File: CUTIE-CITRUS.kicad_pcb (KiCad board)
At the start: 2 copper layers, 78.5 x 78.5 mm, 72 parts, among them J1 F32Q-1A7H1-11022, J2 F32Q-1A7H1-11022, J3 Bus_M.2_Socket_M, P1 ERM8-025-01-L-D-RA-K-TR, U1 AP3441SHE-7B, U2 ASEK-32.768KHZ-L-R-T, U3 ICM-42688-P, U5 MCP98243, U6 MCP98243, U7 MCP2518FD-xQBB, U8 TCAN334

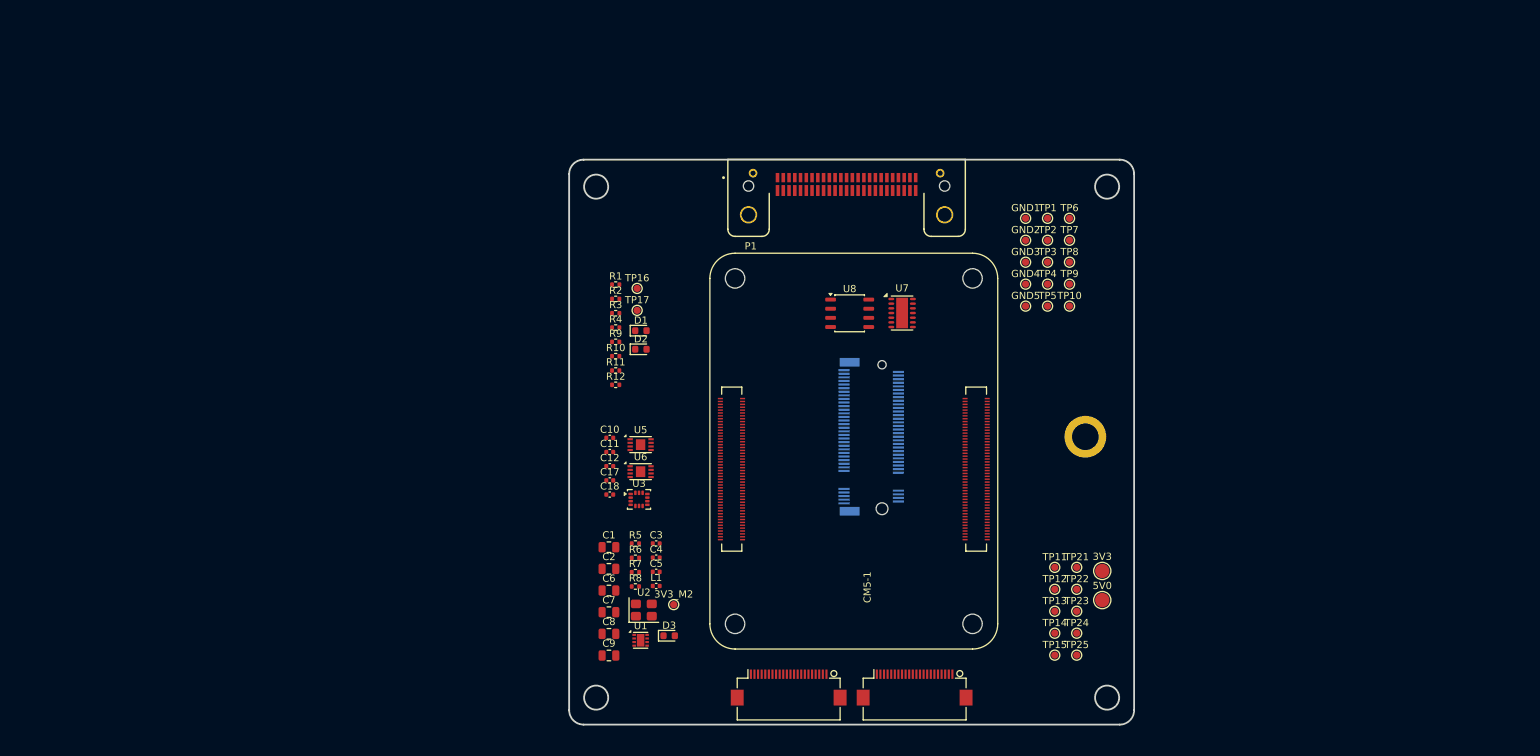
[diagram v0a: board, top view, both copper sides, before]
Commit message: starting layout
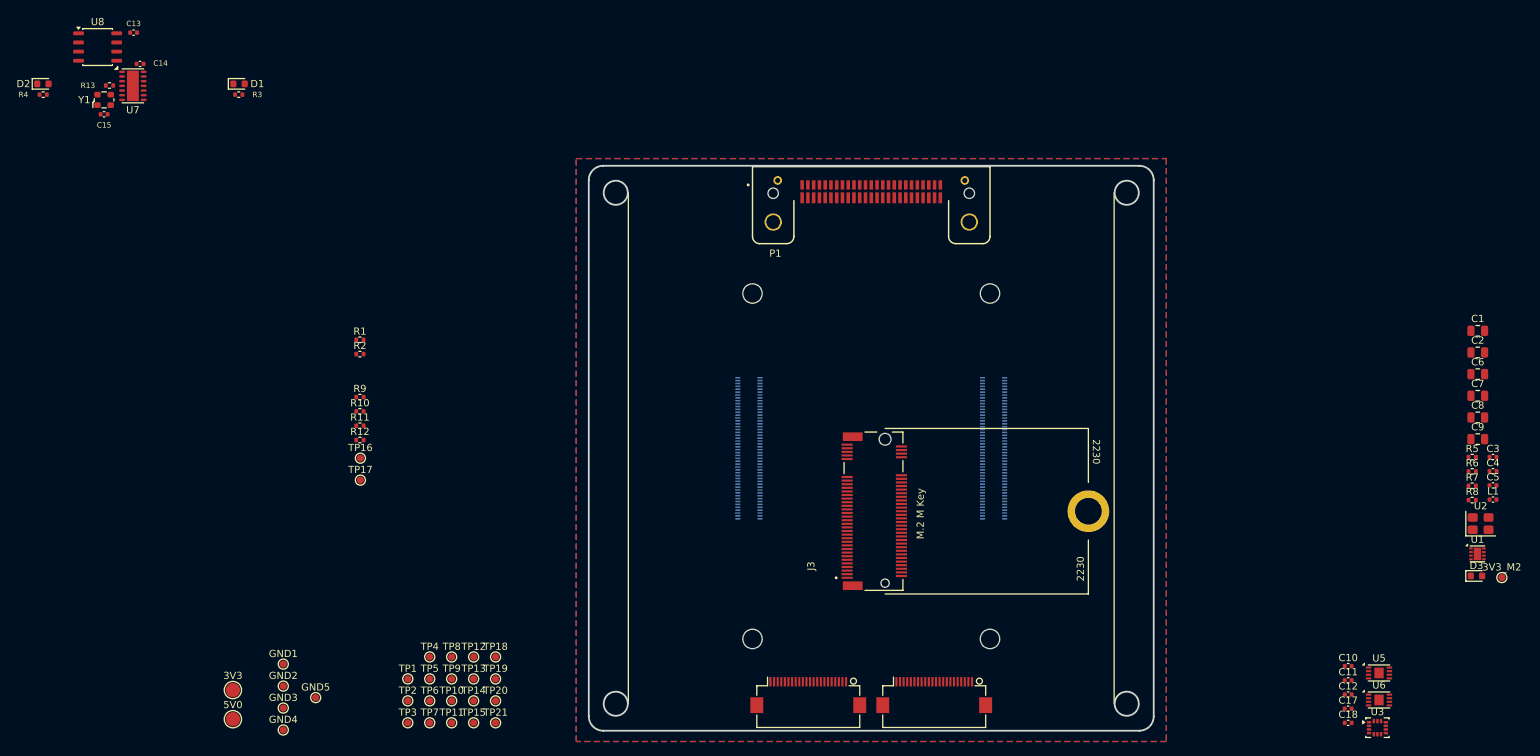
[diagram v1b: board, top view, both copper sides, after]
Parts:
- removed TP22, TP23, TP24, TP25: TestPoint, TestPoint:TestPoint_Pad_D1.0mm
- added C13: 0.1uF, Capacitor_SMD:C_0402_1005Metric, F.Cu at (47.5, 38.5)
- added C14: 0.1uF, Capacitor_SMD:C_0402_1005Metric, F.Cu at (48.4, 42.8)
- added C15: 0.1uF, Capacitor_SMD:C_0402_1005Metric, F.Cu at (43.4, 49.8)
- added R13: 2.2K 1%, Resistor_SMD:R_0402_1005Metric, F.Cu at (44.1, 45.8)
- added TP18: TestPoint, TestPoint:TestPoint_Pad_D1.0mm, F.Cu at (97.8, 125.2)
- added TP19: TestPoint, TestPoint:TestPoint_Pad_D1.0mm, F.Cu at (97.8, 128.3)
- added TP20: TestPoint, TestPoint:TestPoint_Pad_D1.0mm, F.Cu at (97.8, 131.3)
- added Y1: ECS-2520MV-200-BN-TR, Oscillator:Oscillator_SMD_ECS_2520MV-xxx-xx-4Pin_2.5x2.0mm, F.Cu at (43.4, 47.8)
- CM5-1: moved to B.Cu
- J3: moved to F.Cu
- moved C1 124.4 mm to (234.3, 79.9)
- moved C2 124.4 mm to (234.3, 82.9)
- moved C6 124.4 mm to (234.3, 86.0)
- moved C7 124.4 mm to (234.3, 89.0)
- moved C8 124.4 mm to (234.3, 92.0)
- moved C9 124.4 mm to (234.3, 95.0)
- moved 3V3 121.9 mm to (61.3, 129.8)
- moved 5V0 121.9 mm to (61.3, 133.9)
- moved GND2 120.3 mm to (68.3, 129.3)
- moved GND1 120.3 mm to (68.3, 126.2)
- moved GND3 120.3 mm to (68.3, 132.3)
- moved GND4 120.3 mm to (68.3, 135.4)
- moved C3 116.9 mm to (236.4, 97.5)
- moved C4 116.9 mm to (236.4, 99.4)
- moved C5 116.9 mm to (236.4, 101.4)
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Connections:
- net Net-(U7-RXCAN) renamed /CM5/RXCAN
- net Net-(U7-TXCAN) renamed /CM5/TXCAN
- 3V3 pad 1: /Cameras/3V3 -> /CM5/3V3
- C10 pad 1: /Cameras/3V3 -> /CM5/3V3
- C11 pad 1: /Cameras/3V3 -> /CM5/3V3
- C12 pad 1: /Cameras/3V3 -> /CM5/3V3
- C17 pad 1: /Cameras/3V3 -> /CM5/3V3
- C18 pad 1: /Cameras/3V3 -> /CM5/3V3
- CM5-1 pad 128: unconnected-(CM5-1B-USB3-0-RX_N-Pad128) -> /Backplane Connector/USB3.RX_N
- CM5-1 pad 130: unconnected-(CM5-1B-USB3-0-RX_P-Pad130) -> /Backplane Connector/USB3.RX_P
- CM5-1 pad 134: unconnected-(CM5-1B-USB3-0-D_P-Pad134) -> /Backplane Connector/USB3.D_P
- CM5-1 pad 136: unconnected-(CM5-1B-USB3-0-D_N-Pad136) -> /Backplane Connector/USB3.D_N
- CM5-1 pad 140: unconnected-(CM5-1B-USB3-0-TX_N-Pad140) -> /Backplane Connector/USB3.TX_N
- CM5-1 pad 142: unconnected-(CM5-1B-USB3-0-TX_P-Pad142) -> /Backplane Connector/USB3.TX_P
- CM5-1 pad 157: /Backplane Connector/USB3.RX_N -> unconnected-(CM5-1B-USB3-1-RX_N-Pad157)
- CM5-1 pad 159: /Backplane Connector/USB3.RX_P -> unconnected-(CM5-1B-USB3-1-RX_P-Pad159)
- CM5-1 pad 163: /Backplane Connector/USB3.D_P -> unconnected-(CM5-1B-USB3-1-D_P-Pad163)
- CM5-1 pad 165: /Backplane Connector/USB3.D_N -> unconnected-(CM5-1B-USB3-1-D_N-Pad165)
- CM5-1 pad 169: /Backplane Connector/USB3.TX_N -> unconnected-(CM5-1B-USB3-1-TX_N-Pad169)
- CM5-1 pad 171: /Backplane Connector/USB3.TX_P -> unconnected-(CM5-1B-USB3-1-TX_P-Pad171)
- CM5-1 pad 194: GND -> /CM5/DPHY1.D3_N
- CM5-1 pad 196: GND -> /CM5/DPHY1.D3_P
- CM5-1 pad 25: unconnected-(CM5-1A-GPIO21-Pad25) -> /CM5/SPI1.SCLK
- CM5-1 pad 26: unconnected-(CM5-1A-GPIO19-Pad26) -> /CM5/SPI1.MISO
- CM5-1 pad 27: unconnected-(CM5-1A-GPIO20-Pad27) -> /CM5/SPI1.MOSI
- CM5-1 pad 28: unconnected-(CM5-1A-GPIO13-Pad28) -> /CM5/I2C2.SDA
- CM5-1 pad 30: unconnected-(CM5-1A-GPIO6-Pad30) -> /CM5/GPIO/SPI3.MOSI
- CM5-1 pad 31: unconnected-(CM5-1A-GPIO12-Pad31) -> /CM5/I2C2.SDA
- CM5-1 pad 34: /CM5/I2C2.SCL -> /CM5/GPIO/SPI3.MISO
- CM5-1 pad 35: /CM5/I2C1.SCL -> /Backplane Connector/SPI2.MISO
- CM5-1 pad 36: /CM5/I2C1.SDA -> /Backplane Connector/SPI2.CS0n
- CM5-1 pad 37: /CM5/SPI0.CS1n -> /CM5/GPIO/SPI3.SCLK
- CM5-1 pad 38: /CM5/SPI0.SCLK -> /CM5/I2C1.SCL
- CM5-1 pad 39: /CM5/SPI0.CS0n -> /CM5/I2C0.SDA
- CM5-1 pad 40: /CM5/SPI0.MISO -> /CM5/I2C0.SCL
- CM5-1 pad 41: unconnected-(CM5-1A-GPIO25-Pad41) -> /CM5/CAN_INT
- CM5-1 pad 44: /CM5/SPI0.MOSI -> /CM5/I2C1.SDA
- CM5-1 pad 49: unconnected-(CM5-1A-GPIO18-Pad49) -> /CM5/SPI1.CS0n
- CM5-1 pad 50: unconnected-(CM5-1A-GPIO17-Pad50) -> /CM5/SPI1.CS1n
- CM5-1 pad 54: /CM5/I2C2.SDA -> /CM5/GPIO/SPI3.CS0n
- CM5-1 pad 56: unconnected-(CM5-1A-GPIO3-Pad56) -> /Backplane Connector/SPI2.SCLK
- CM5-1 pad 58: unconnected-(CM5-1A-GPIO2-Pad58) -> /Backplane Connector/SPI2.MOSI
- CM5-1 pad 78: /Cameras/3V3 -> /CM5/3V3
- CM5-1 pad 80: /CM5/I2C0.SCL -> unconnected-(CM5-1A-GPIO39-Pad80)
- CM5-1 pad 82: /CM5/I2C0.SDA -> unconnected-(CM5-1A-GPIO38-Pad82)
- CM5-1 pad 84: /Cameras/3V3 -> /CM5/3V3
- CM5-1 pad 86: /Cameras/3V3 -> /CM5/3V3
- D1 pad 2: /Cameras/3V3 -> /CM5/3V3
- D2 pad 2: /Cameras/3V3 -> /CM5/3V3
- J1 pad 22: /Cameras/3V3 -> /CM5/3V3
- J2 pad 22: /Cameras/3V3 -> /CM5/3V3
- P1 pad 01: (no net) -> /Backplane Connector/CAN0.L
- P1 pad 02: (no net) -> GND
- P1 pad 03: (no net) -> /Backplane Connector/CAN0.H
- P1 pad 04: (no net) -> GND
- P1 pad 05: (no net) -> GND
- P1 pad 06: (no net) -> /Backplane Connector/USB3.D_N
- P1 pad 07: (no net) -> GND
- P1 pad 08: (no net) -> /Backplane Connector/USB3.D_P
- P1 pad 09: (no net) -> unconnected-(P1-Pad09)
- P1 pad 30: /Backplane Connector/SPI1.MOSI -> /Backplane Connector/SPI2.MOSI
- P1 pad 32: /Backplane Connector/SPI1.MISO -> /Backplane Connector/SPI2.MISO
- P1 pad 38: /Backplane Connector/SPI1.SCLK -> /Backplane Connector/SPI2.SCLK
- P1 pad 40: /Backplane Connector/SPI1.CS0n -> /Backplane Connector/SPI2.CS0n
- R1 pad 1: /Cameras/3V3 -> /CM5/3V3
- R10 pad 1: /Cameras/3V3 -> /CM5/3V3
- R11 pad 1: /Cameras/3V3 -> /CM5/3V3
- R12 pad 1: /Cameras/3V3 -> /CM5/3V3
- R2 pad 1: /Cameras/3V3 -> /CM5/3V3
- R9 pad 1: /Cameras/3V3 -> /CM5/3V3
- TP1 pad 1: /CM5/SPI0.MISO -> /CM5/PCIEsb.nCLKREQ
- TP10 pad 1: /CM5/I2C2.SDA -> /CM5/I2C2.SCL
- TP11 pad 1: /CM5/I2C2.SCL -> /CM5/SPI1.MISO
- TP12 pad 1: /CM5/PCIEsb.nCLKREQ -> /CM5/SPI1.MOSI
- TP13 pad 1: /CM5/PCIEsb.nWAKE -> /CM5/SPI1.SCLK
- TP14 pad 1: /CM5/PCIEsb.PWR_EN -> /CM5/SPI1.CS0n
- TP15 pad 1: /CM5/PCIEsb.nRST -> /CM5/SPI1.CS1n
- TP2 pad 1: /CM5/SPI0.MOSI -> /CM5/PCIEsb.nWAKE
- TP21 pad 1: /Backplane Connector/SPI1.MISO -> /Backplane Connector/SPI2.CS0n
- TP3 pad 1: /CM5/SPI0.SCLK -> /CM5/PCIEsb.PWR_EN
- TP4 pad 1: /CM5/SPI0.CS0n -> /CM5/PCIEsb.nRST
- TP5 pad 1: /CM5/SPI0.CS1n -> /CM5/I2C0.SDA
- TP6 pad 1: /CM5/I2C0.SDA -> /CM5/I2C0.SCL
- TP7 pad 1: /CM5/I2C0.SCL -> /CM5/I2C1.SDA
- TP8 pad 1: /CM5/I2C1.SDA -> /CM5/I2C1.SCL
- TP9 pad 1: /CM5/I2C1.SCL -> /CM5/I2C2.SDA
- U3 pad 1: /CM5/SPI0.MISO -> /CM5/SPI1.MISO
- U3 pad 12: /CM5/SPI0.CS0n -> /CM5/SPI1.CS0n
- U3 pad 13: /CM5/SPI0.SCLK -> /CM5/SPI1.SCLK
- U3 pad 14: /CM5/SPI0.MOSI -> /CM5/SPI1.MOSI
- U3 pad 5: /Cameras/3V3 -> /CM5/3V3
- U3 pad 8: /Cameras/3V3 -> /CM5/3V3
- U5 pad 8: /Cameras/3V3 -> /CM5/3V3
- U6 pad 1: /Cameras/3V3 -> /CM5/3V3
- U6 pad 8: /Cameras/3V3 -> /CM5/3V3
- U7 pad 10: /CM5/SPI4.SCLK -> /CM5/GPIO/SPI3.SCLK
- U7 pad 11: /CM5/SPI4.MOSI -> /CM5/GPIO/SPI3.MOSI
- U7 pad 12: /CM5/SPI4.MISO -> /CM5/GPIO/SPI3.MISO
- U7 pad 13: /CM5/SPI4.CS0n -> /CM5/GPIO/SPI3.CS0n
- U7 pad 14: unconnected-(U7-VDD-Pad14) -> /CM5/3V3
- U7 pad 15: unconnected-(U7-VSS-Pad15) -> GND
- U7 pad 4: unconnected-(U7-~{INT}-Pad4) -> /CM5/CAN_INT
- U7 pad 6: unconnected-(U7-OSC1-Pad6) -> /CM5/OSC1
- U7 pad 7: unconnected-(U7-VSS-Pad7) -> GND
- U8 pad 2: unconnected-(U8-GND-Pad2) -> GND
- U8 pad 3: unconnected-(U8-VCC-Pad3) -> /CM5/3V3
- U8 pad 5: unconnected-(U8-SHDN-Pad5) -> GND
- U8 pad 8: unconnected-(U8-STB-Pad8) -> /CM5/3V3
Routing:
- added copper zone on B.Cu, net GND
- added copper zone on F.Cu, net GND
- added copper zone on In1.Cu, net GND
- added copper zone on In2.Cu, net GND
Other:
- copper layers 2 -> 4
- board text removed: "For Instructional Use Only."
- board text removed: "SOLIDWORKS Educational Product."
